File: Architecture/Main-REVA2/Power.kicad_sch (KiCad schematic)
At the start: 39 parts, among them J7 1.8 - 5.5 - Battery, J8 12V - Secteur, U1 MIC4690

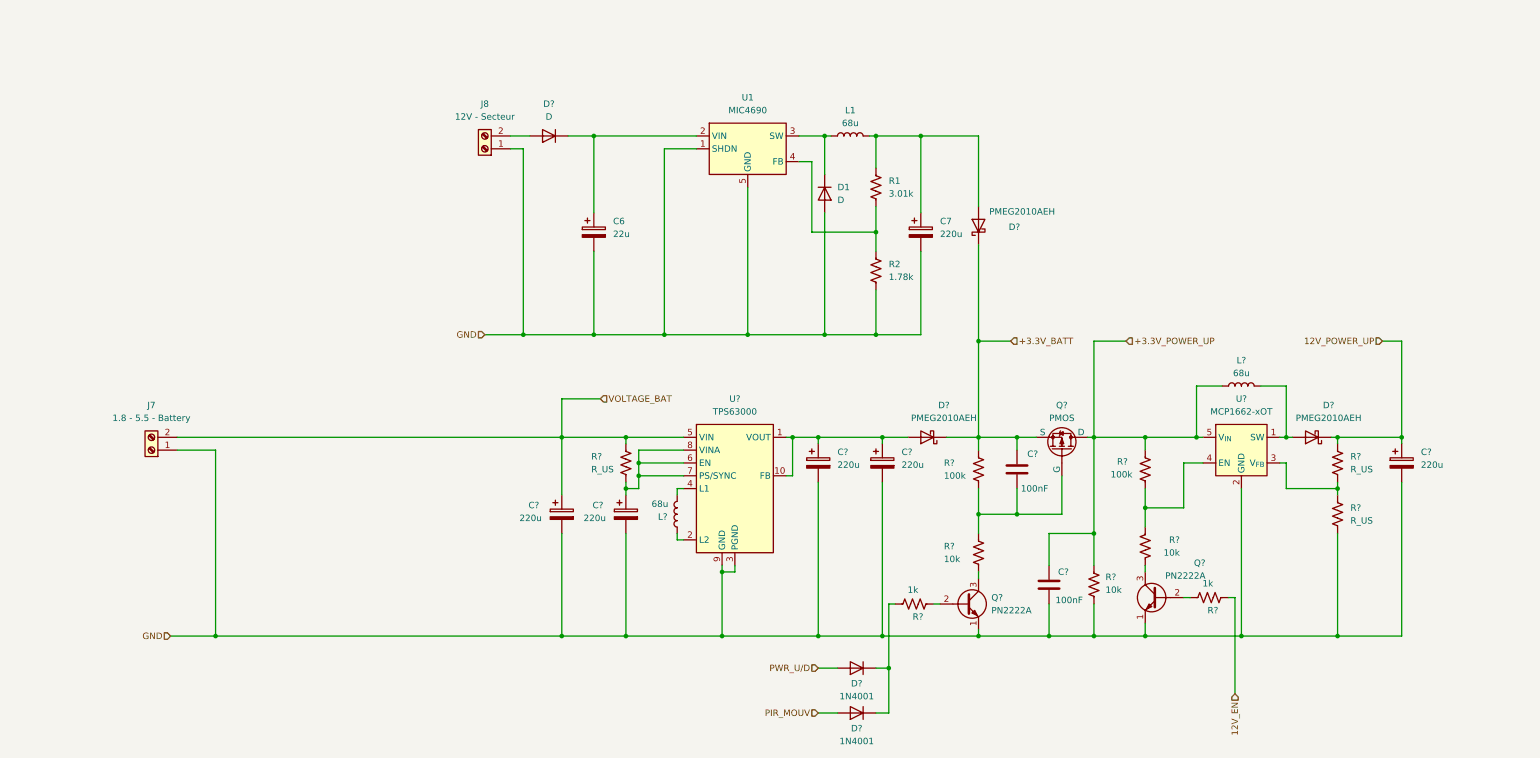
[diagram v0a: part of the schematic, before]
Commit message: Update_Schematic
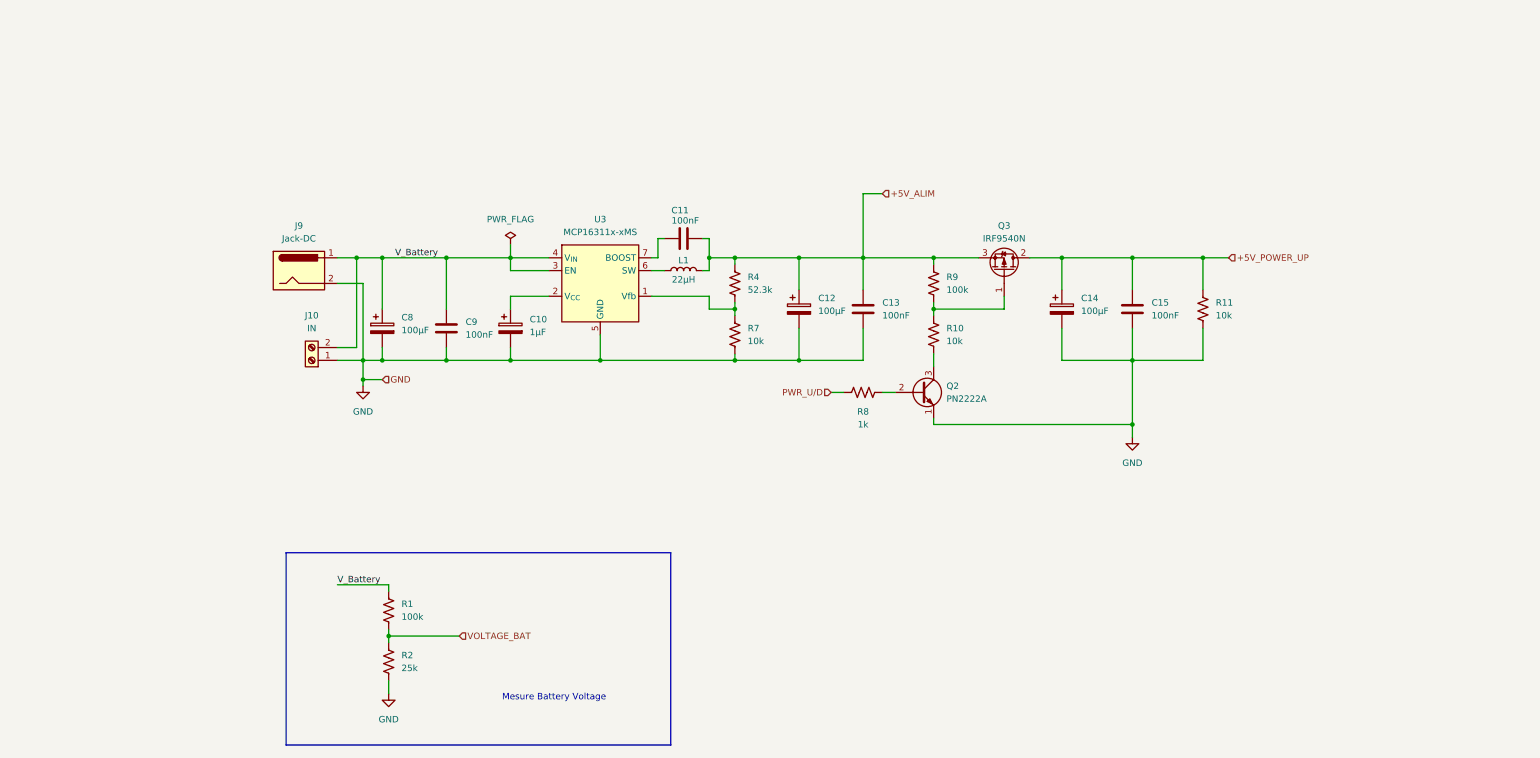
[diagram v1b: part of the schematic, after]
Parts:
- removed C6: 22u, symbol Device:C_Polarized
- removed C7, C? (x5): 220u, symbol Device:C_Polarized
- removed C? (x2): 100nF, symbol Device:C
- removed D1, D?: D, symbol Device:D
- removed D? (x2): 1N4001, Diode_THT:D_DO-41_SOD81_P10.16mm_Horizontal, symbol Diode:1N4001
- removed D? (x3): PMEG2010AEH, Diode_SMD:D_SOD-123F, symbol Diode:PMEG2010AEH
- removed J7: 1.8 - 5.5 - Battery, symbol Connector:Screw_Terminal_01x02
- removed J8: 12V - Secteur, symbol Connector:Screw_Terminal_01x02
- removed L? (x2): 68u, symbol Device:L
- removed Q?: PMOS, symbol Simulation_SPICE:PMOS
- removed Q? (x2): PN2222A, Package_TO_SOT_THT:TO-92_Inline, symbol Transistor_BJT:PN2222A
- removed R? (x2): 1k, symbol Device:R_US
- removed R? (x3): 10k, symbol Device:R_US
- removed R? (x3): R_US, symbol Device:R_US
- removed R? (x2): 100k, symbol Device:R_US
- removed U1: MIC4690, Package_SO:SOIC-8_3.9x4.9mm_P1.27mm, symbol Regulator_Switching:MIC4690
- removed U?: TPS63000, Package_SON:Texas_DRC0010J_ThermalVias, symbol Regulator_Switching:TPS63000
- removed U?: MCP1662-xOT, Package_TO_SOT_SMD:SOT-23-5, symbol Driver_LED:MCP1662-xOT
- added C10: 1µF, symbol Device:C_Polarized
- added C11, C13, C15, C9: 100nF, symbol Device:C
- added C12, C14, C8: 100µF, symbol Device:C_Polarized
- added J10: IN, symbol Connector:Screw_Terminal_01x02
- added J9: Jack-DC, symbol Connector:Jack-DC
- added Q2: PN2222A, Package_TO_SOT_THT:TO-92_Inline, symbol Transistor_BJT:PN2222A
- added Q3: IRF9540N, Package_TO_SOT_THT:TO-220-3_Vertical, symbol Transistor_FET:IRF9540N
- added R10, R11, R7: 10k, symbol Device:R_US
- added R4: 52.3k, symbol Device:R_US
- added R8: 1k, symbol Device:R_US
- added R9: 100k, symbol Device:R_US
- added U3: MCP16311x-xMS, Package_SO:MSOP-8_3x3mm_P0.65mm, symbol Regulator_Switching:MCP16311x-xMS
- L1: value 68u -> 22µH
- R1: value 3.01k -> 100k
- R2: value 1.78k -> 25k
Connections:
- net GND: now also C10.2, C12.2, C13.2, C14.2, C15.2, C8.2, C9.2, J10.1 (Pin_1), J9.2, Q2.1 (E), R11.2, R7.2, U3.5 (GND), U3.8 (GND)
- net PWR_U/D: now also R8.1
- net VOLTAGE_BAT: now also R1.2, R2.1
- net at L1.1: now also U3.6 (SW)
- net +5V_ALIM: now reaches L1.2
- net +5V_ALIM: now also C11.2, C12.1, C13.1, Q3.3 (S), R4.1, R9.1; no longer R1.1
- new net: C10.1, U3.2 (V_{CC})
- new net: Q3.1 (G), R10.1, R9.2
- new net: R4.2, R7.1, U3.1 (Vfb)
- new net: C11.1, U3.7 (BOOST)
- new net: Q2.3 (C), R10.2
- new net: Q2.2 (B), R8.2
- new net +5V_POWER_UP: C14.1, C15.1, Q3.2 (D), R11.1
- new net V_Battery: C8.1, C9.1, J10.2 (Pin_2), J9.1, R1.1, U3.3 (EN), U3.4 (V_{IN})
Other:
- note added: "Mesure Battery Voltage"
- company: (none) -> Polytech Nantes - ETN4
- title: (none) -> Collecteur de données Animalières
